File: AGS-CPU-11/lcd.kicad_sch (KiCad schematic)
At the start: 56 parts, among them P2 LCD, Q12 DTA114T, Q7 DTA114T, SW2 LIGHT ON, U6 NL17SZ74, U8 XP04501

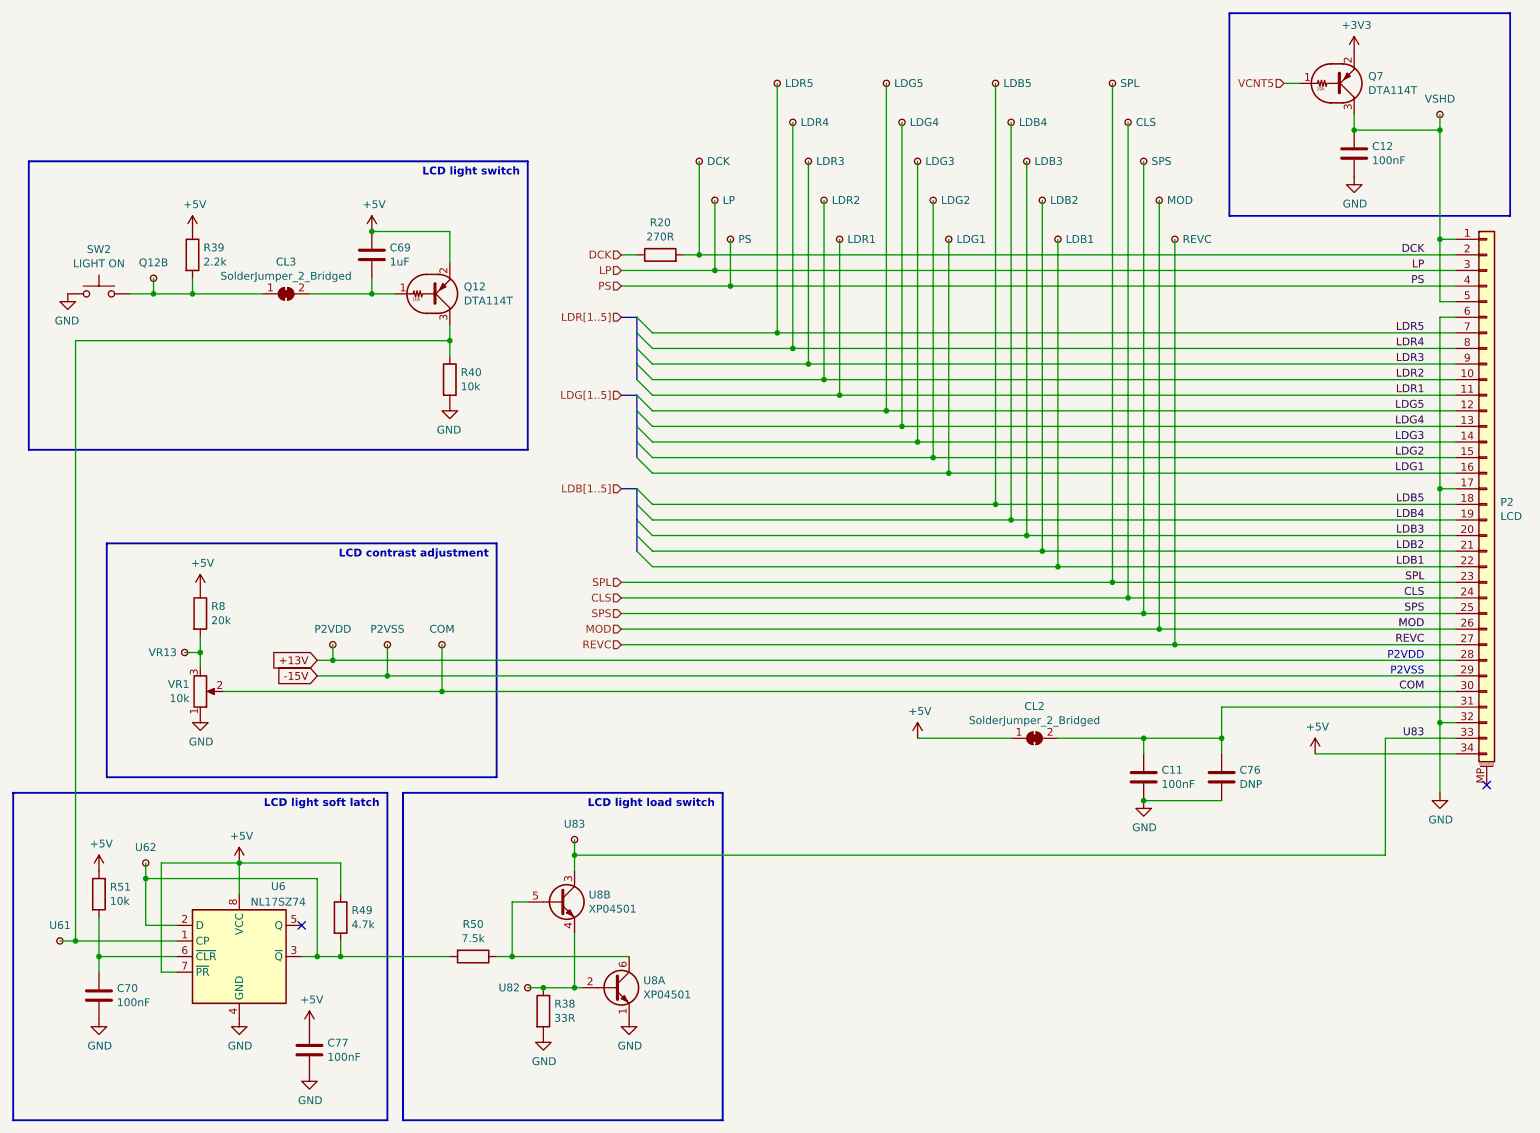
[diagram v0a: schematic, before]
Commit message: Update to latest KiCad
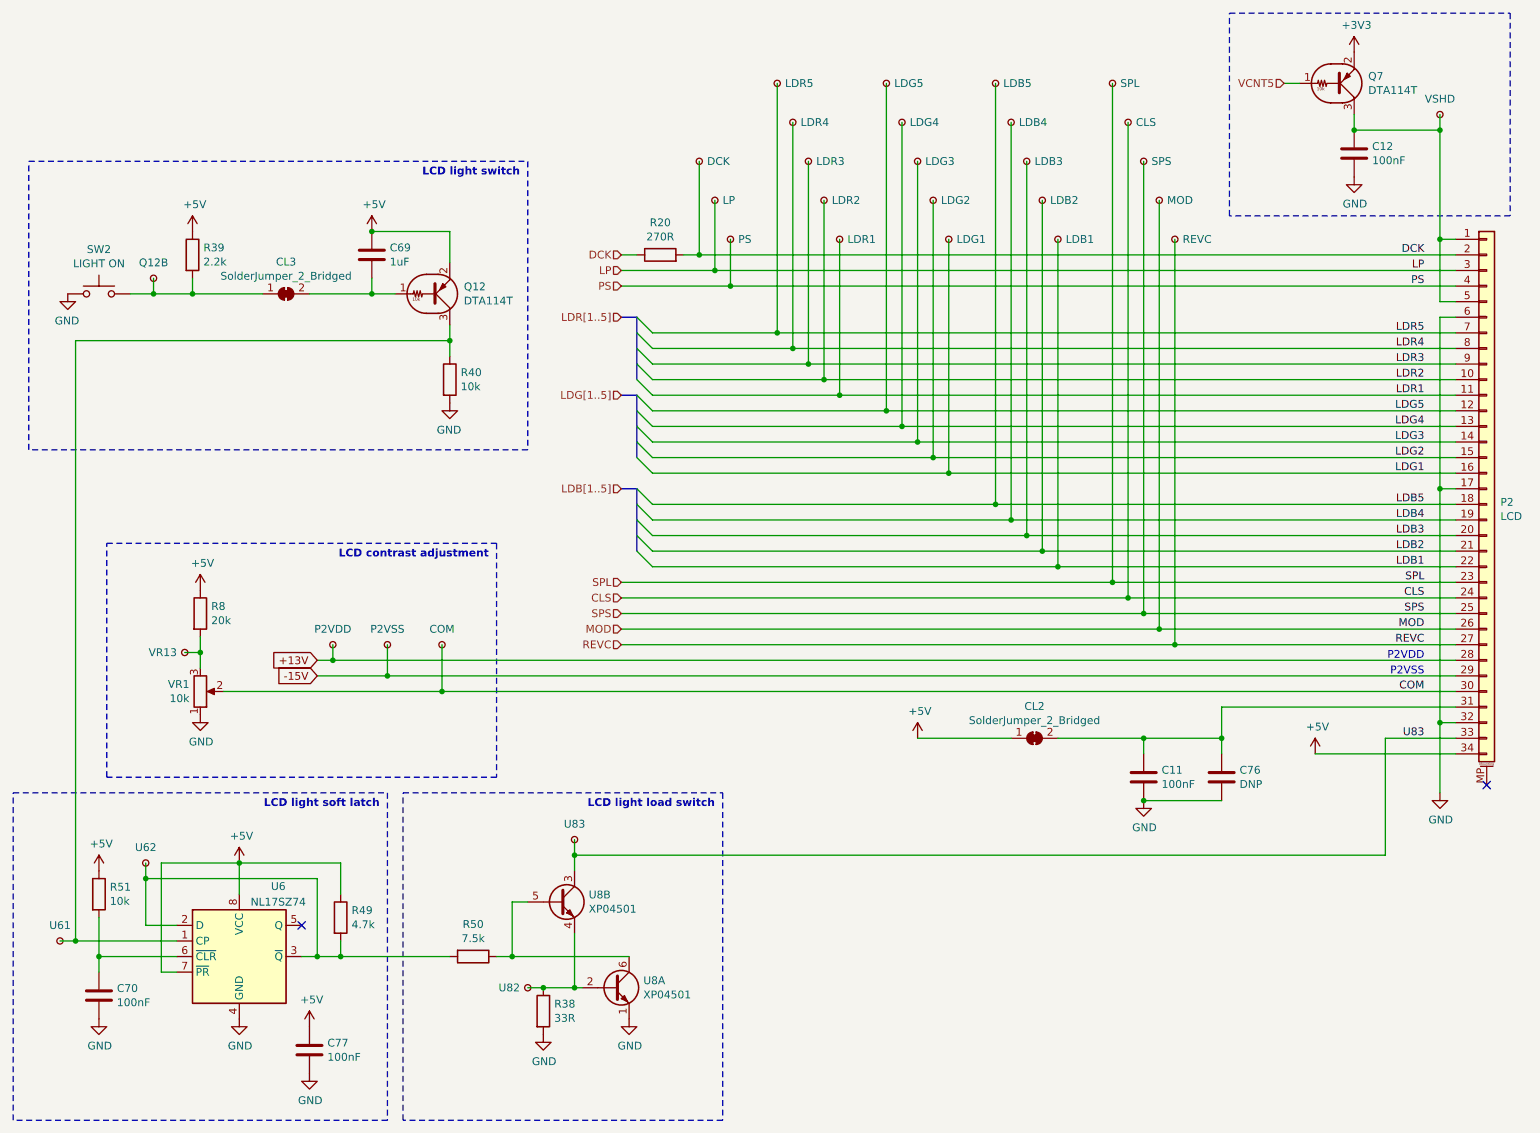
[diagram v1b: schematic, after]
